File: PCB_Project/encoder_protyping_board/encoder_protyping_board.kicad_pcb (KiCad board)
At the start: 2 copper layers, 24.3 x 21.6 mm, 11 parts, among them J1 Conn_02x04_Counter_Clockwise, J2 Conn_01x02_Pin, J3 Conn_01x03_Pin

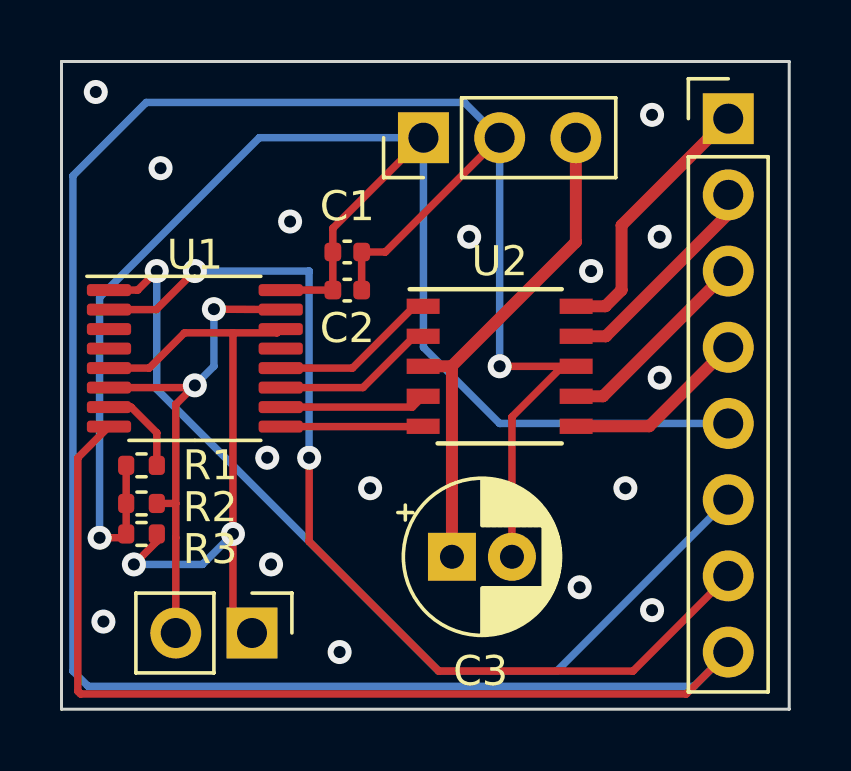
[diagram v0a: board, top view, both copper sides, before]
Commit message: manual routing is fun
it is basically a puzzle
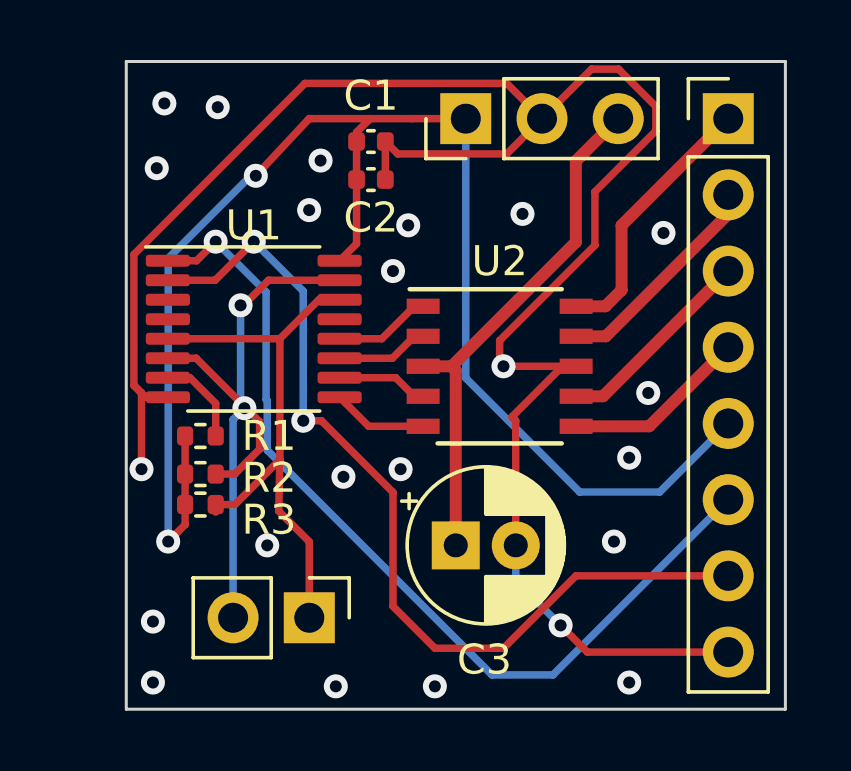
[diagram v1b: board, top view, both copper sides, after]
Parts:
- moved C1 3.77 mm to (64.3, 17.9)
- moved C2 3.77 mm to (64.3, 19.2)
- moved R1 2.19 mm to (58.6, 27.7)
- moved R2 2.19 mm to (58.6, 29.0)
- moved U1 2.19 mm to (60.4, 24.2)
- moved R3 2.19 mm to (58.6, 30.0)
- moved J2 1.98 mm to (62.2, 33.8)
- moved J3 1.55 mm to (67.5, 17.1)
- moved C3 0.40 mm to (67.1, 31.4)
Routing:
- net GND: track 111.4 -> 66.9 mm, vias 17 -> 23
- net I2C_SDA: track 17.1 -> 21.1 mm
- net Net-(J1-Pin_7): track 33.4 -> 30.6 mm
- net I2C_SCL: track 21.6 -> 19.1 mm, vias 2 -> 0
- net Net-(U1-OUT1): track 5.46 -> 3.09 mm
- net Net-(U1-OUT0): track 5.60 -> 3.23 mm
- net Net-(U1-OUT2): track 4.90 -> 3.04 mm
- net Net-(U1-OUT3): track 4.75 -> 3.20 mm
- net +12V: track 17.4 -> 18.3 mm
- net Net-(J1-Pin_6): track 31.1 -> 30.4 mm
- net +5V: track 50.6 -> 51.1 mm, vias 1 -> 2
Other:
- board size 24.3 x 21.6 mm -> 22 x 21.6 mm
